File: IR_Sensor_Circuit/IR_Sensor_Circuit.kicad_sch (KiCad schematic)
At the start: 8 parts, among them J1 Conn_01x03_Pin, U1 LM358

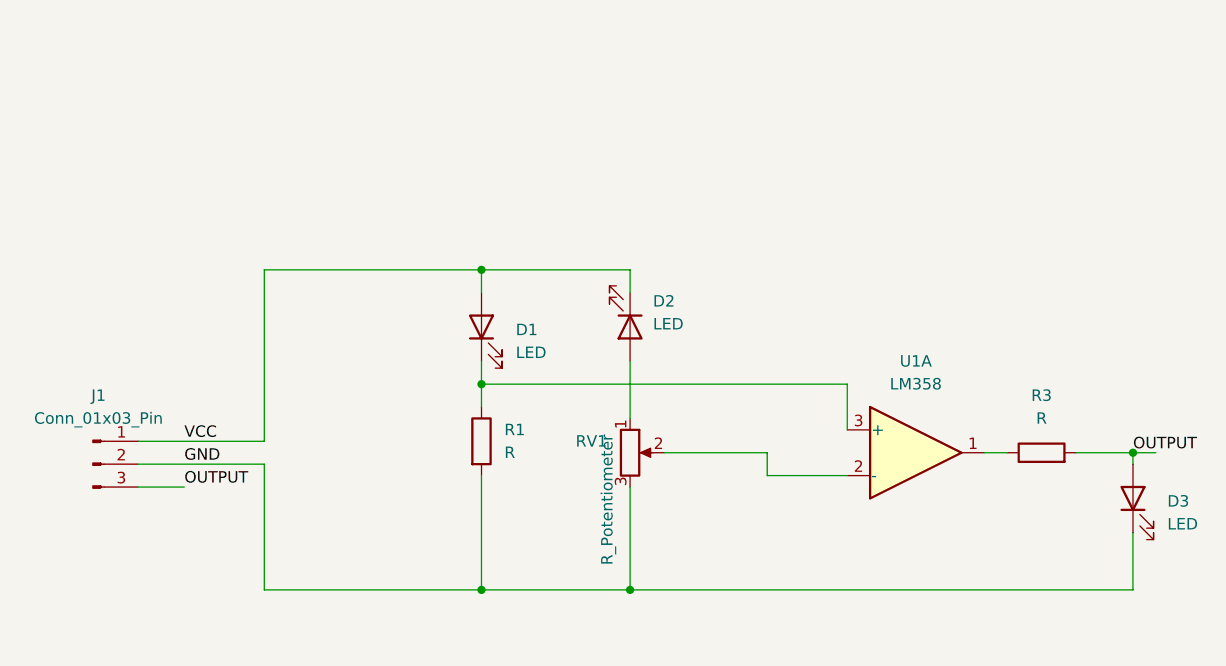
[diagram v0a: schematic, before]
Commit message: IR Circuit
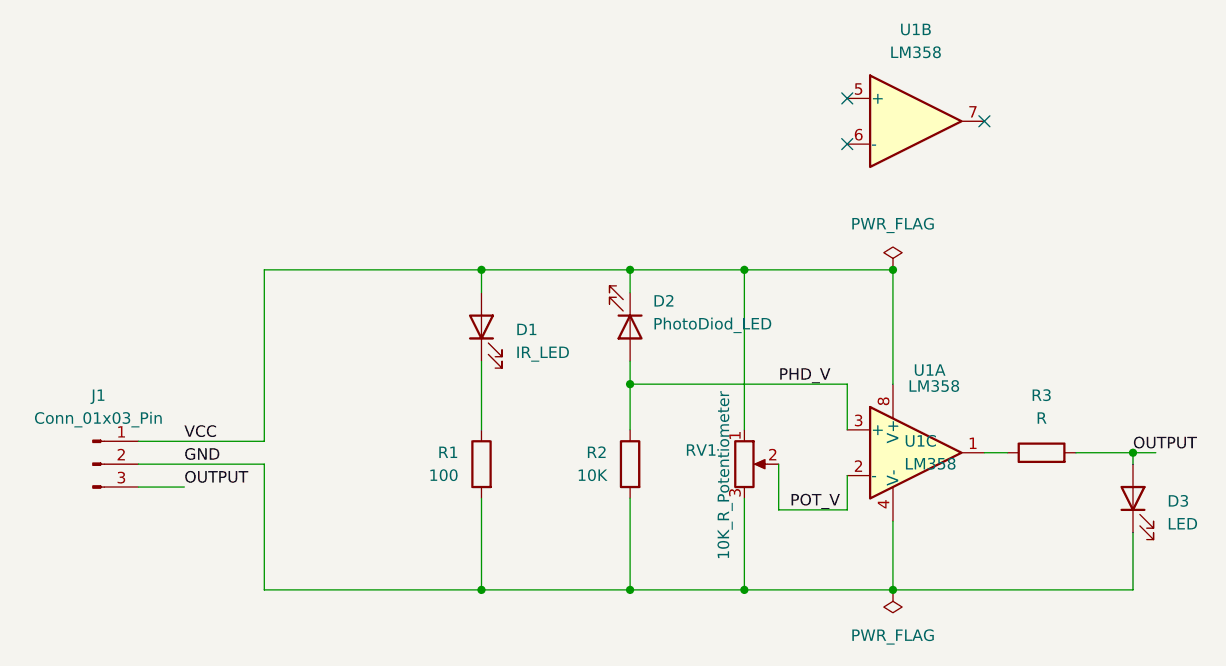
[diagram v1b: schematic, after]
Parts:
- added R2: 10K, Resistor_SMD:R_1206_3216Metric, symbol Device:R
- added unit 2 of U1
- added unit 3 of U1
- D1: value LED -> IR_LED; footprint (none) -> LED_SMD:LED_1206_3216Metric
- D2: value LED -> PhotoDiod_LED; footprint (none) -> LED_SMD:LED_1206_3216Metric
- D3: footprint (none) -> LED_SMD:LED_1206_3216Metric
- J1: footprint (none) -> Connector_PinHeader_2.54mm:PinHeader_1x03_P2.54mm_Horizontal
- R1: value R -> 100; footprint (none) -> Resistor_SMD:R_1206_3216Metric
- R3: footprint (none) -> Resistor_SMD:R_1206_3216Metric
- RV1: value R_Potentiometer -> 10K_R_Potentiometer; footprint (none) -> Potentiometer_SMD:Potentiometer_Bourns_3314J_Vertical
- U1: footprint (none) -> Package_TO_SOT_SMD:SOT-23-8
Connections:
- net GND: now also R2.2, U1.4 (V-)
- net VCC: now also RV1.1, U1.8 (V+)
- net POT_V: now reaches RV1.2, U1.2 (-)
- net at D1.1 (K), R1.1: no longer U1.3 (+)
- net PHD_V: now reaches D2.2 (A)
- net PHD_V: now also U1.3 (+), R2.1; no longer RV1.1
- no-connect marks 0 -> 3
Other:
- moved on the sheet: R1
